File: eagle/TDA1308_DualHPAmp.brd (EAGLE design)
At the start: 33.1 x 66.1 mm, 28 parts, among them IC1 TDA1308, IC2 TDA1308

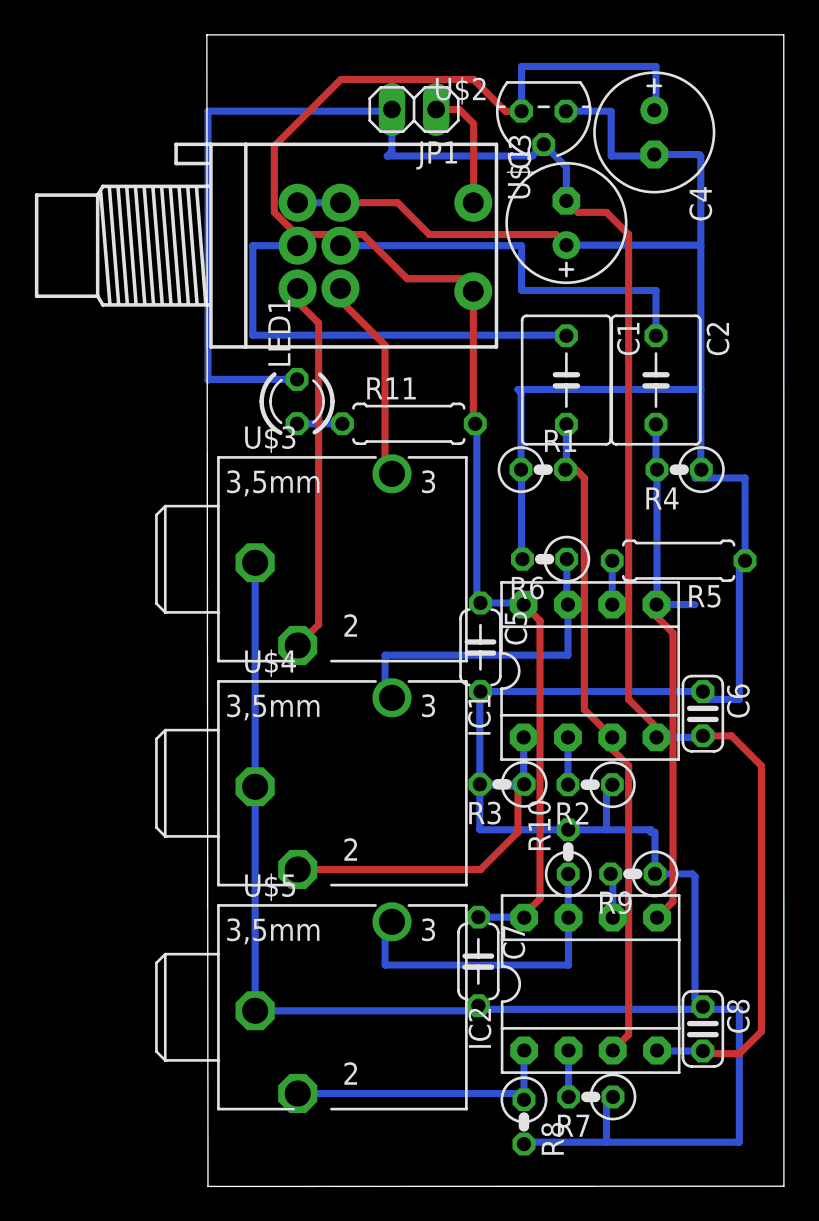
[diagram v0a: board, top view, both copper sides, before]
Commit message: Update
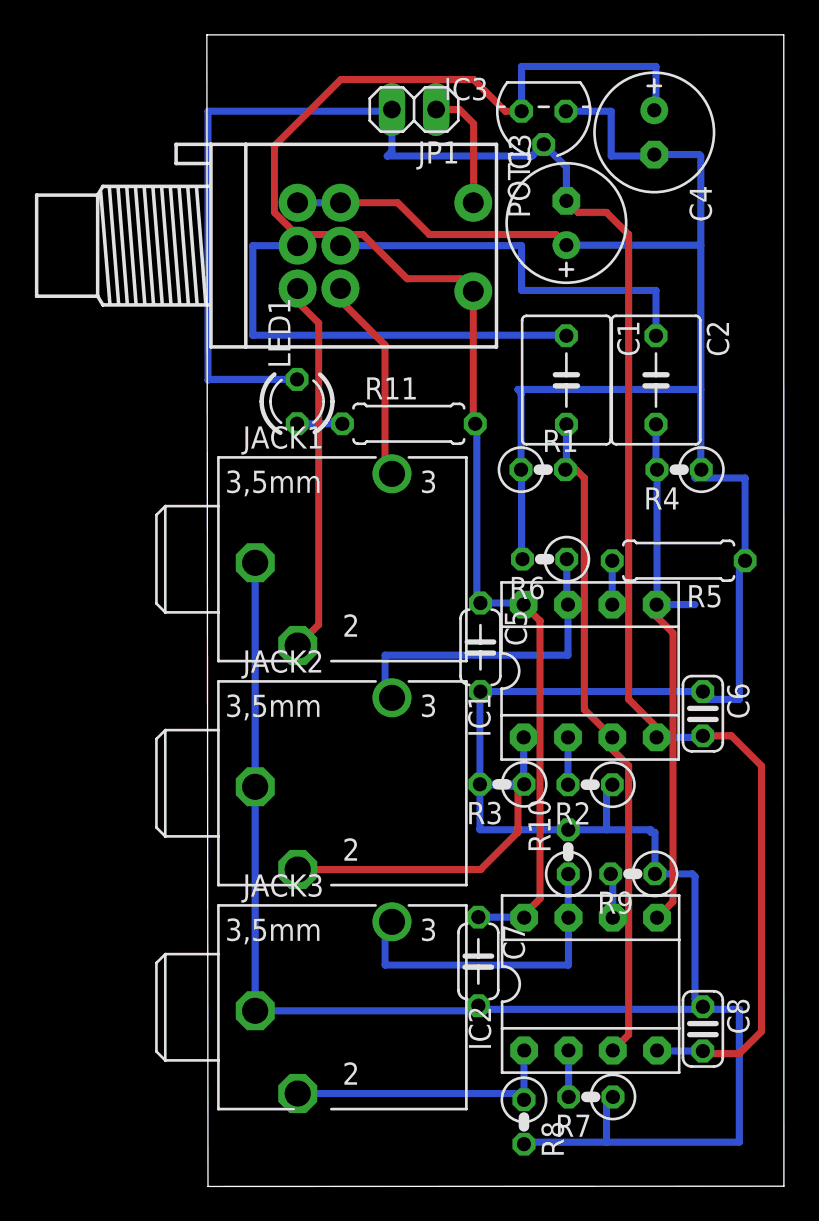
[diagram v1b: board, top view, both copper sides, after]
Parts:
- C2: value (none) -> 1uF
- R4: value 1uF -> 100k
- renumbered U$1 to POT1, U$2 to IC3, U$3 to JACK1, U$4 to JACK2, U$5 to JACK3
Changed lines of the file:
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@@
 <elements>
 <element name="C1" library="rcl" package="C050-050X075" value="1uF" x="20.56" y="46.26" rot="R270"/>
-<element name="C2" library="rcl" package="C050-050X075" value="" x="25.7" y="46.26" rot="R270"/>
+<element name="C2" library="rcl" package="C050-050X075" value="1uF" x="25.7" y="46.26" rot="R270"/>
 <element name="R1" library="rcl" package="0207/2V" value="100k" x="19.23" y="41.12"/>
-<element name="R4" library="rcl" package="0207/2V" value="1uF" x="27.03" y="41.12" rot="R180"/>
+<element name="R4" library="rcl" package="0207/2V" value="100k" x="27.03" y="41.12" rot="R180"/>
 <element name="IC1" library="burr-brown" package="DIL08" value="TDA1308" x="21.92" y="29.57">
 <attribute name="OC_NEWARK" value="74K3897" x="21.92" y="29.57" size="1.778" layer="27" display="off"/>
@@
 <element name="R11" library="rcl" package="0207/7" value="6.8k" x="11.52" y="43.75"/>
 <element name="LED1" library="led" package="LED3MM" value="Blue" x="5.110675" y="45.025459375" rot="R90"/>
-<element name="U$2" library="tle2426" package="TO226AA" value="TLE2426CLP" x="19.26" y="61.68" rot="R180"/>
+<element name="IC3" library="tle2426" package="TO226AA" value="TLE2426CLP" x="19.26" y="61.68" rot="R180"/>
 <element name="C3" library="rcl" package="E2,5-7" value="100u" x="20.56" y="55.27" rot="R90"/>
 <element name="C4" library="rcl" package="E2,5-7" value="100u" x="25.600615625" y="60.466315625" rot="R270"/>
@@
 <element name="C7" library="rcl" package="C050-024X044" value="0.1u" x="15.51" y="12.91" rot="R270"/>
 <element name="C8" library="rcl" package="C025-024X044" value="0.1u" x="28.39" y="9.04" rot="R270"/>
-<element name="U$1" library="mylib2" package="RK0971221" value="RK0971221" x="5.14" y="53.97" rot="R270"/>
-<element name="U$3" library="mylib2" package="MJ-3052W-0" value="MJ-353W-0" x="7.71" y="35.98"/>
-<element name="U$4" library="mylib2" package="MJ-3052W-0" value="MJ-353W-0" x="7.71" y="23.13"/>
-<element name="U$5" library="mylib2" package="MJ-3052W-0" value="MJ-353W-0" x="7.71" y="10.28"/>
+<element name="POT1" library="mylib2" package="RK0971221" value="RK0971221" x="5.14" y="53.97" rot="R270"/>
+<element name="JACK1" library="mylib2" package="MJ-3052W-0" value="MJ-353W-0" x="7.71" y="35.98"/>
+<element name="JACK2" library="mylib2" package="MJ-3052W-0" value="MJ-353W-0" x="7.71" y="23.13"/>
+<element name="JACK3" library="mylib2" package="MJ-3052W-0" value="MJ-353W-0" x="7.71" y="10.28"/>
 </elements>
 <signals>
 <signal name="N$1">
-<contactref element="U$1" pad="1-3"/>
-<contactref element="U$3" pad="2"/>
+<contactref element="POT1" pad="1-3"/>
+<contactref element="JACK1" pad="2"/>
 <wire x1="5.14" y1="51.51" x2="5.14" y2="50.74" width="0.4064" layer="1"/>
 <wire x1="5.14" y1="50.74" x2="6.35" y2="49.53" width="0.4064" layer="1"/>
@@
 </signal>
 <signal name="N$2">
-<contactref element="U$1" pad="2-3"/>
-<contactref element="U$3" pad="3"/>
+<contactref element="POT1" pad="2-3"/>
+<contactref element="JACK1" pad="3"/>
 <wire x1="7.6" y1="51.51" x2="7.6" y2="50.82" width="0.4064" layer="1"/>
 <wire x1="7.6" y1="50.82" x2="10.16" y2="48.26" width="0.4064" layer="1"/>
@@
 <contactref element="R9" pad="1"/>
 <contactref element="R10" pad="2"/>
-<contactref element="U$1" pad="1-1"/>
-<contactref element="U$1" pad="2-1"/>
-<contactref element="U$3" pad="1"/>
-<contactref element="U$4" pad="1"/>
-<contactref element="U$5" pad="1"/>
+<contactref element="POT1" pad="1-1"/>
+<contactref element="POT1" pad="2-1"/>
+<contactref element="JACK1" pad="1"/>
+<contactref element="JACK2" pad="1"/>
+<contactref element="JACK3" pad="1"/>
 <contactref element="C5" pad="2"/>
 <contactref element="C3" pad="+"/>
-<contactref element="U$2" pad="1"/>
+<contactref element="IC3" pad="1"/>
 <contactref element="C8" pad="1"/>
 <contactref element="C6" pad="1"/>
@@
 <signal name="N$3">
 <contactref element="C1" pad="1"/>
-<contactref element="U$1" pad="1-2"/>
+<contactref element="POT1" pad="1-2"/>
 <wire x1="5.14" y1="53.97" x2="2.57" y2="53.97" width="0.4064" layer="16"/>
 <wire x1="2.57" y1="53.97" x2="2.57" y2="48.83" width="0.4064" layer="16"/>
@@
 <signal name="N$4">
 <contactref element="C2" pad="1"/>
-<contactref element="U$1" pad="2-2"/>
+<contactref element="POT1" pad="2-2"/>
 <wire x1="7.6" y1="53.97" x2="17.99" y2="53.97" width="0.4064" layer="16"/>
 <wire x1="17.99" y1="53.97" x2="17.99" y2="51.4" width="0.4064" layer="16"/>
@@
 <contactref element="IC1" pad="1"/>
 <contactref element="R3" pad="1"/>
-<contactref element="U$4" pad="2"/>
+<contactref element="JACK2" pad="2"/>
 <wire x1="18.136984375" y1="23.0698625" x2="18.11" y2="23.0698625" width="0.4064" layer="16"/>
 <wire x1="18.11" y1="23.0698625" x2="18.11" y2="25.76" width="0.4064" layer="16"/>
@@
 <contactref element="LED1" pad="K"/>
 <contactref element="C6" pad="2"/>
-<contactref element="U$2" pad="2"/>
+<contactref element="IC3" pad="2"/>
 <contactref element="JP1" pad="2"/>
 <contactref element="C8" pad="2"/>
@@
 <contactref element="IC1" pad="8"/>
 <contactref element="IC2" pad="8"/>
-<contactref element="U$2" pad="3"/>
+<contactref element="IC3" pad="3"/>
 <contactref element="R11" pad="2"/>
 <contactref element="C5" pad="1"/>
 <contactref element="C7" pad="1"/>
 <contactref element="C4" pad="+"/>
-<contactref element="U$1" pad="3-2"/>
+<contactref element="POT1" pad="3-2"/>
 <wire x1="17.99" y1="61.68" x2="17.99" y2="64.25" width="0.4064" layer="16"/>
 <wire x1="17.99" y1="64.25" x2="25.7" y2="64.25" width="0.4064" layer="16"/>
@@
 <contactref element="IC1" pad="7"/>
 <contactref element="R6" pad="1"/>
-<contactref element="U$4" pad="3"/>
+<contactref element="JACK2" pad="3"/>
 <wire x1="20.65" y1="33.38" x2="20.581509375" y2="33.38" width="0.4064" layer="16"/>
 <wire x1="20.581509375" y1="33.38" x2="20.581509375" y2="35.98429375" width="0.4064" layer="16"/>
@@
 <contactref element="IC2" pad="1"/>
 <contactref element="R8" pad="1"/>
-<contactref element="U$5" pad="2"/>
+<contactref element="JACK3" pad="2"/>
 <wire x1="18.14" y1="7.8" x2="18.1258875" y2="7.8" width="0.4064" layer="16"/>
 <wire x1="18.1258875" y1="7.8" x2="18.1258875" y2="4.970959375" width="0.4064" layer="16"/>
@@
 <contactref element="IC2" pad="7"/>
 <contactref element="R10" pad="1"/>
-<contactref element="U$5" pad="3"/>
+<contactref element="JACK3" pad="3"/>
 <wire x1="20.68" y1="15.42" x2="20.32" y2="15.42" width="0.4064" layer="16"/>
 <wire x1="20.32" y1="15.42" x2="20.32" y2="15.24" width="0.4064" layer="16"/>
@@
 <signal name="N$10">
 <contactref element="JP1" pad="1"/>
-<contactref element="U$1" pad="3-1"/>
+<contactref element="POT1" pad="3-1"/>
 <wire x1="13.09" y1="61.78" x2="14.42" y2="61.78" width="0.4064" layer="1"/>
 <wire x1="14.42" y1="61.78" x2="15.24" y2="60.96" width="0.4064" layer="1"/>
